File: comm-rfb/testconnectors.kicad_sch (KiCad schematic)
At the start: 3 parts, among them J10 Conn_02x04_Counter_Clockwise, J11 Conn_02x06_Odd_Even, J12 Conn_02x05_Counter_Clockwise

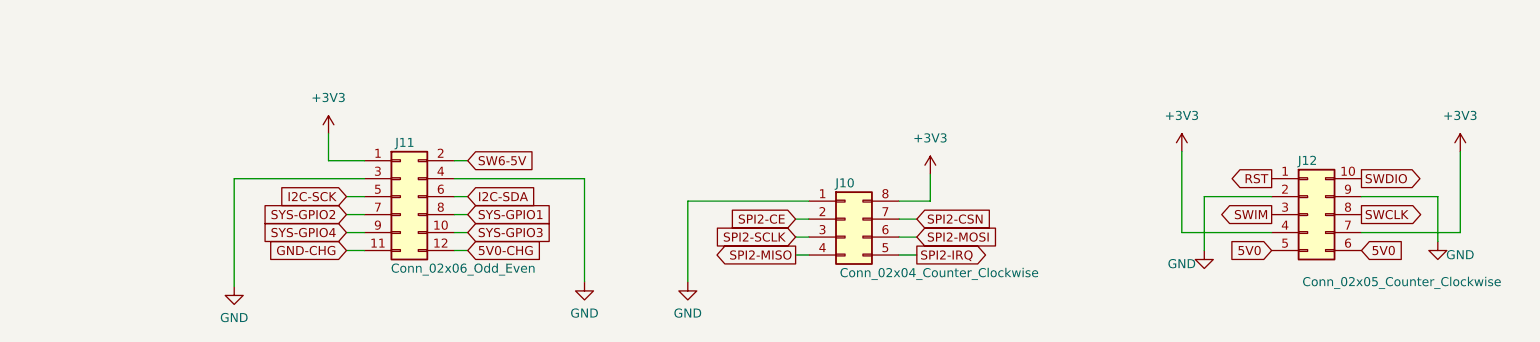
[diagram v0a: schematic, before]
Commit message: comm-rfb: reduce number of sheets in schematic
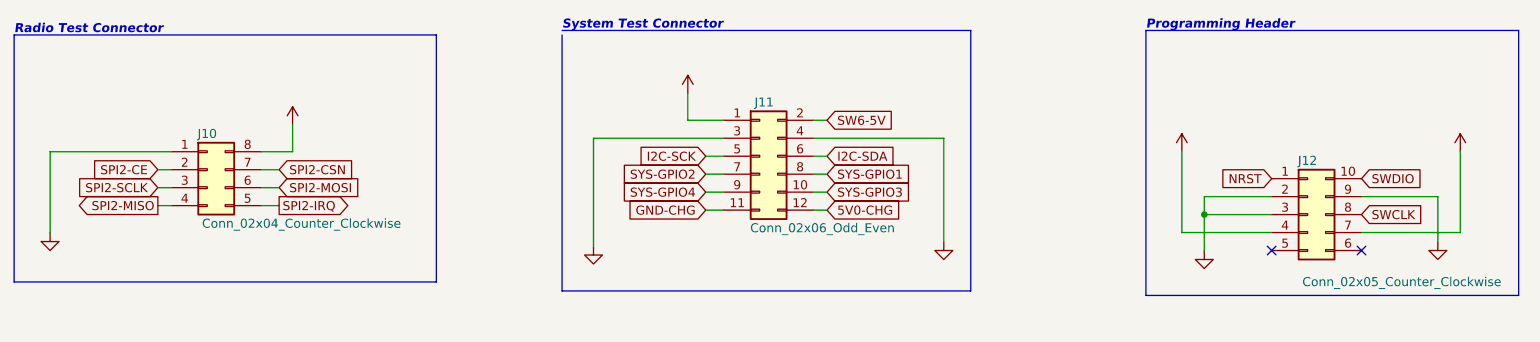
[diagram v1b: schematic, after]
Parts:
- J10: footprint (none) -> Connector_PinSocket_2.54mm:PinSocket_2x04_P2.54mm_Vertical
- J11: footprint (none) -> Connector_PinSocket_2.54mm:PinSocket_2x06_P2.54mm_Horizontal
- J12: footprint (none) -> Connector_PinSocket_2.54mm:PinSocket_2x05_P2.54mm_Horizontal
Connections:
- net SWIM is gone; now on net GND: J12.3 (Pin_3)
- net 5V0: no longer names the net of J12.5 (Pin_5)
- net 5V0: no longer J12.6 (Pin_6)
- net RST renamed NRST
- no-connect marks 0 -> 2
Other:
- note added: "Programming Header"
- note added: "Radio Test Connector"
- note added: "System Test Connector"
- moved on the sheet: J10, J11
